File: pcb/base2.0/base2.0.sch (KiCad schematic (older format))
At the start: 32 parts, among them J1 Conn_01x01_Male, J2 Conn_01x01_Male, J3 Conn_01x04_Male, J4 Conn_01x02_Male, U1 STM32G431CBU6, U2 tile, U3 AP2210-33, U4 MPU-9250

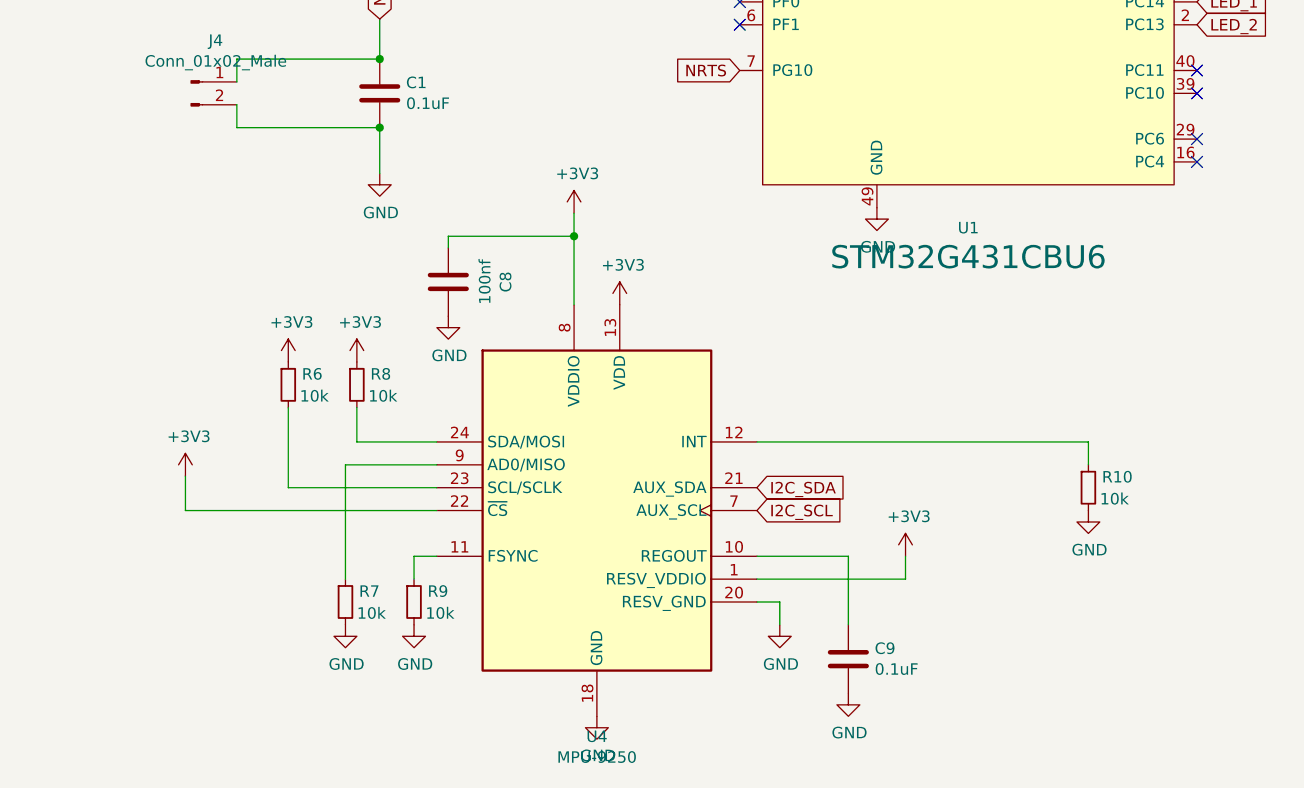
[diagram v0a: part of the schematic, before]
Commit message: le update
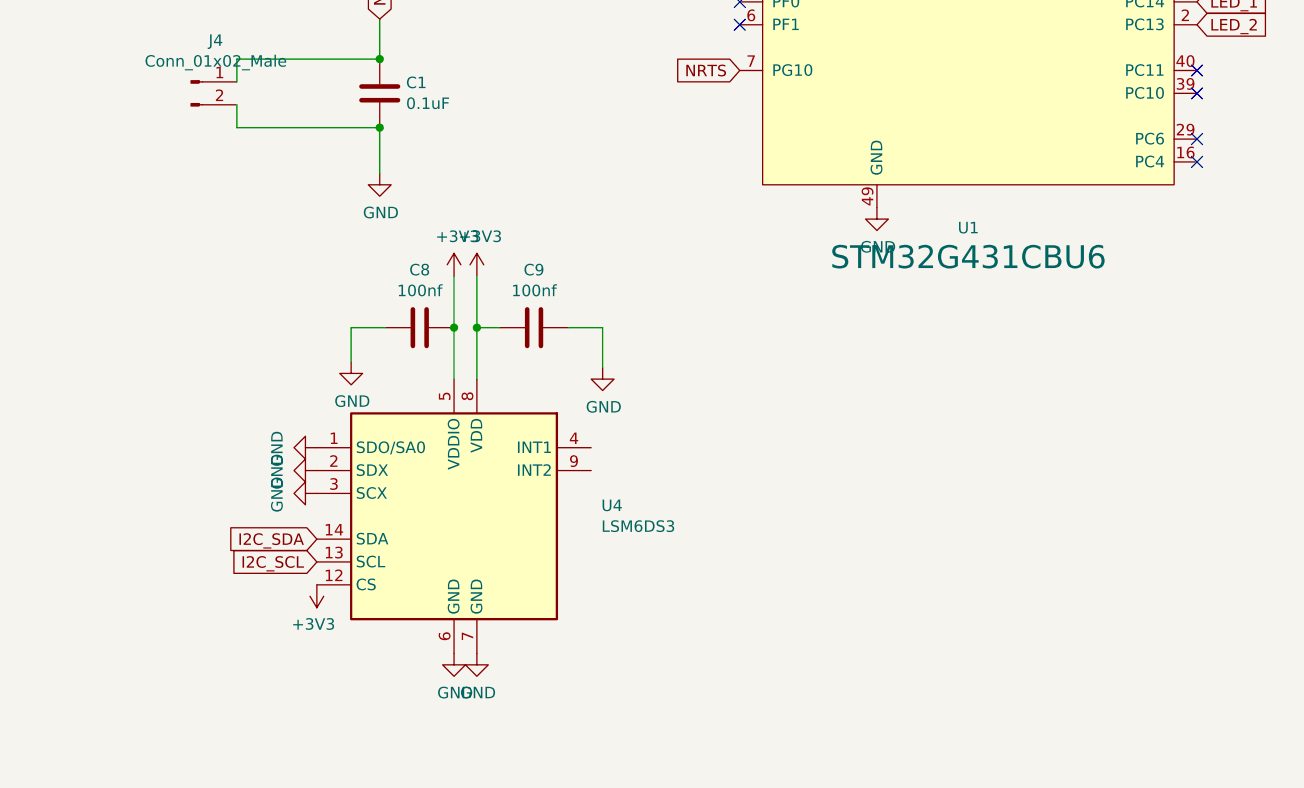
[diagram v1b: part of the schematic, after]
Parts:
- removed R10, R6, R7, R8, R9: 10k, Resistor_SMD:R_0402_1005Metric, symbol Device:R_Small
- removed U4: MPU-9250, Sensor_Motion:InvenSense_QFN-24_3x3mm_P0.4mm, symbol Sensor_Motion:MPU-9250
- added U4: LSM6DS3, Package_LGA:LGA-14_3x2.5mm_P0.5mm_LayoutBorder3x4y, symbol Sensor_Motion:LSM6DS3
- C9: value 0.1uF -> 100nf
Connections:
- net +3V3: now also C8.1, C9.2, U4.12 (CS), U4.5 (VDDIO), U4.8 (VDD); no longer C8.2
- net GND: now also C8.2, C9.1, U4.1 (SDO/SA0), U4.2 (SDX), U4.3 (SCX), U4.6 (GND), U4.7 (GND); no longer C8.1, C9.2
- net I2C_SCL: now also U4.13 (SCL)
- net I2C_SDA: now also U4.14 (SDA)
